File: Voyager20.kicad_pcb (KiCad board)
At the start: 2 copper layers, 73 x 95.2 mm, 92 parts, among them Q1 Q_NPN_BEC, SW1 SW_Push, U1 ATmega32U2-AU, U2 PRTR5V0U2X, Y1 16MHz

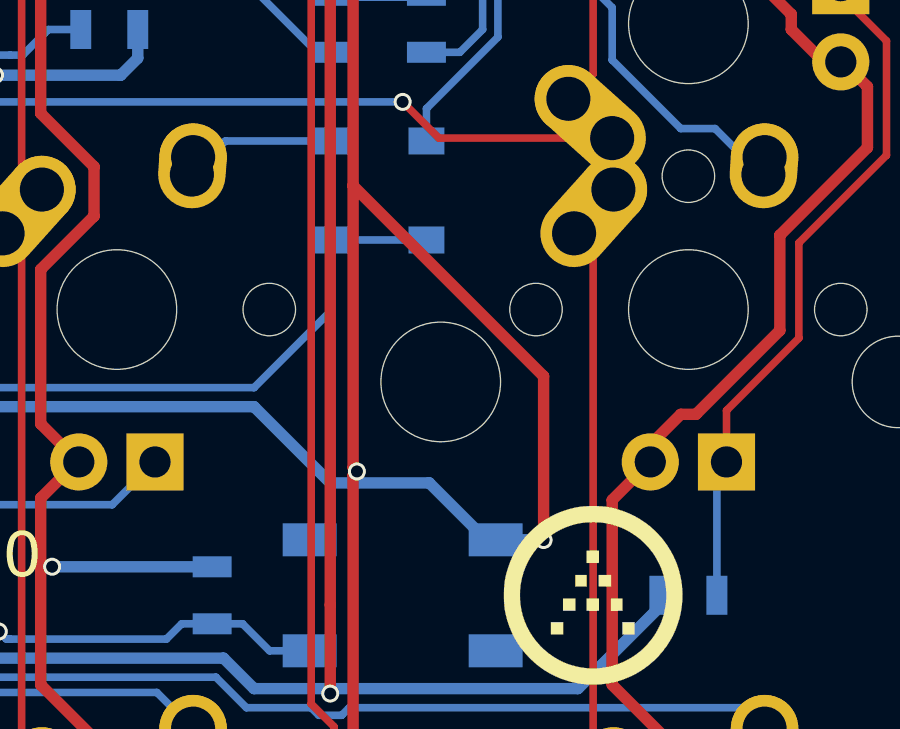
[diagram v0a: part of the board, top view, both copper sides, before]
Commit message: Voyager20 update
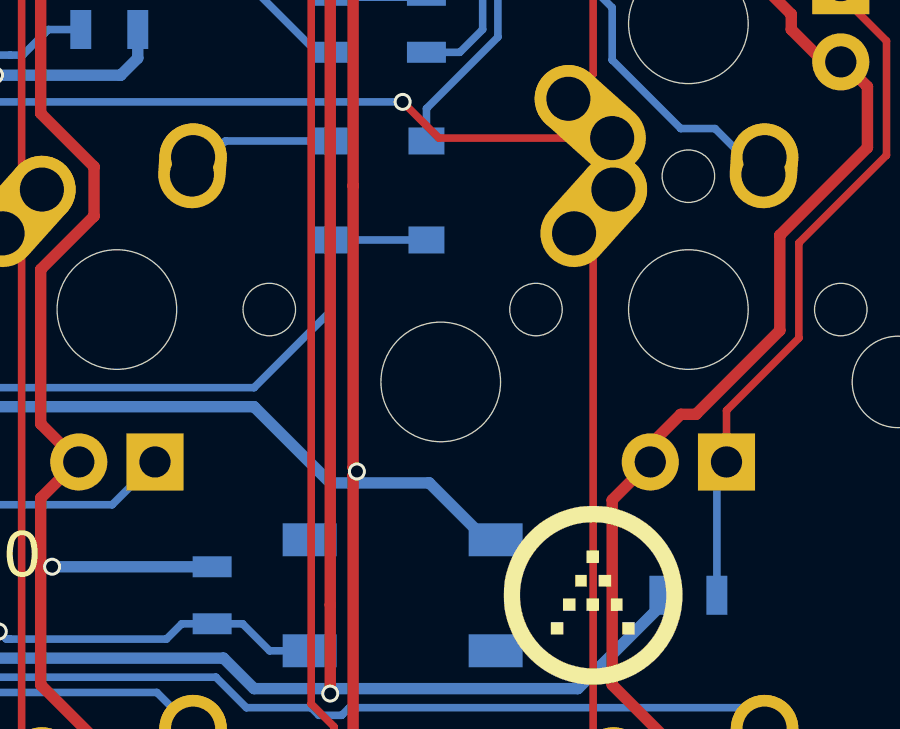
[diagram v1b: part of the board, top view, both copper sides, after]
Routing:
- net GND: track 345.4 -> 329.3 mm, vias 11 -> 10
